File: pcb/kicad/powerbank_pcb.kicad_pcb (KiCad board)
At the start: 2 copper layers, 17.9 x 64.9 mm, 32 parts, among them J1 USB_C_OUT, J2 USB_C_IN, U1 TPS61022, U2 IP2312-ESOP8

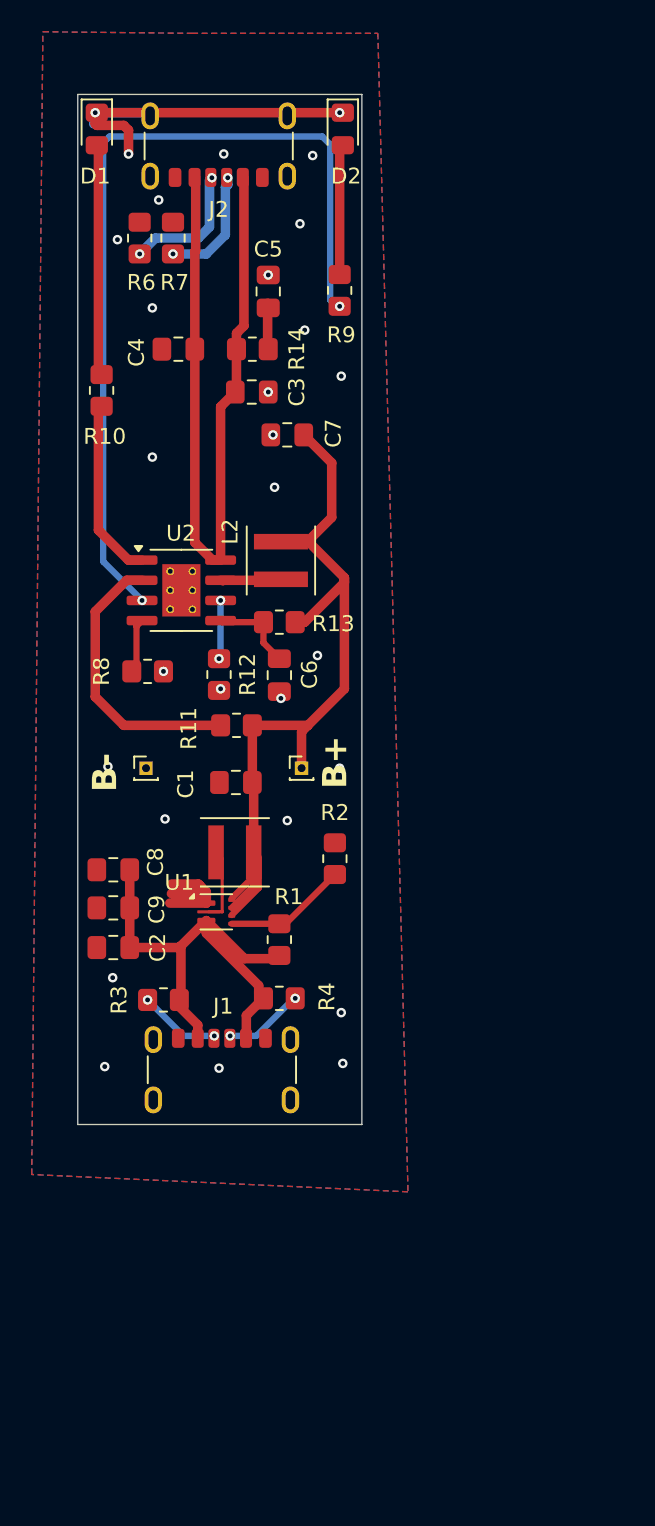
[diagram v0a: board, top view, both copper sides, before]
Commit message: first draft
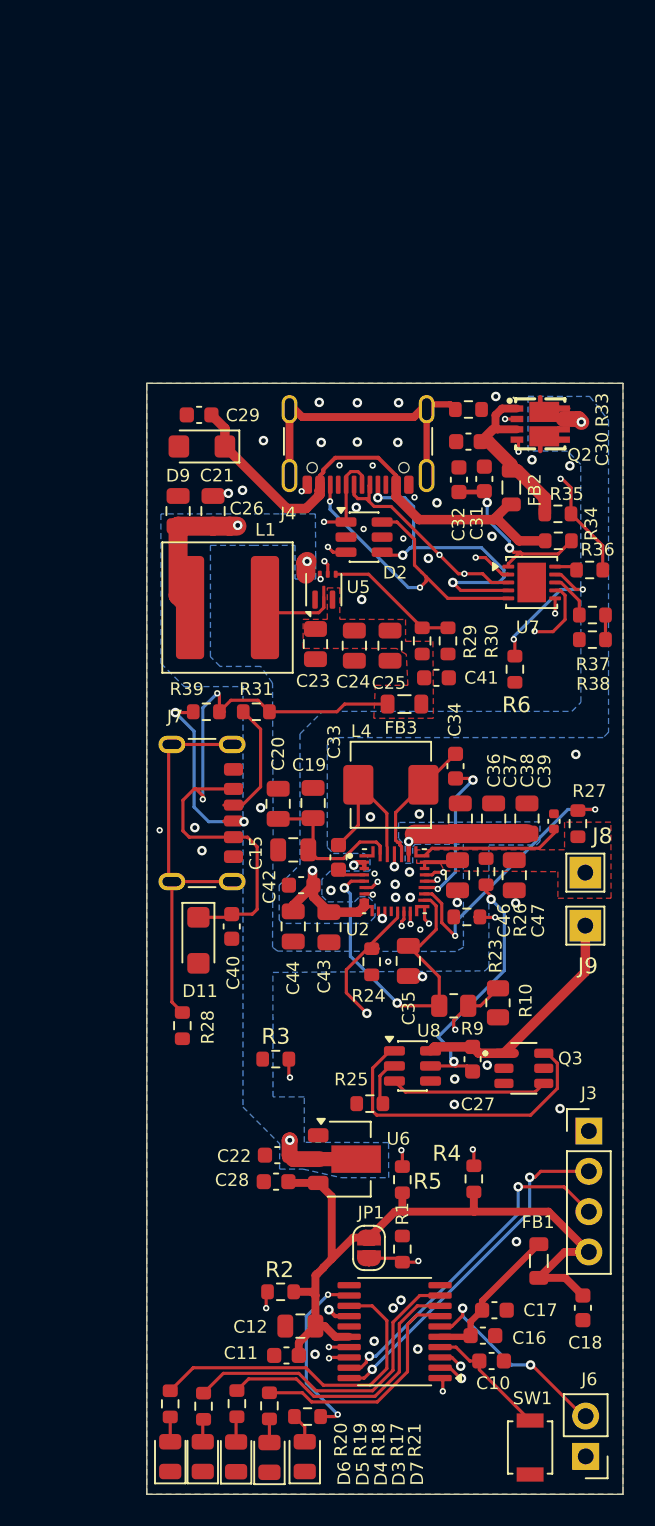
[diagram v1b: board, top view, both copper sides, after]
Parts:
- removed C1, C4, C5: 10uF, Capacitor_SMD:C_0805_2012Metric_Pad1.18x1.45mm_HandSolder
- removed C2, C3, C6, C7, C8, C9: 22uF, Capacitor_SMD:C_0805_2012Metric_Pad1.18x1.45mm_HandSolder
- removed D1: LED_RED, LED_SMD:LED_0805_2012Metric_Pad1.15x1.40mm_HandSolder
- removed J1: USB_C_OUT, Connector_USB:USB_C_Receptacle_GCT_USB4125-xx-x_6P_TopMnt_Horizontal
- removed J2: USB_C_IN, Connector_USB:USB_C_Receptacle_GCT_USB4125-xx-x_6P_TopMnt_Horizontal
- removed L2: 1uH, Inductor_SMD:L_Coilcraft_XxL4030
- removed R11: 1k, Resistor_SMD:R_0805_2012Metric_Pad1.20x1.40mm_HandSolder
- removed R12: 45k, Resistor_SMD:R_0805_2012Metric_Pad1.20x1.40mm_HandSolder
- removed R13: 0.5R, Resistor_SMD:R_0805_2012Metric_Pad1.20x1.40mm_HandSolder
- removed R14: 2R, Resistor_SMD:R_0805_2012Metric_Pad1.20x1.40mm_HandSolder
- removed R7: 5.1k, Resistor_SMD:R_0805_2012Metric_Pad1.20x1.40mm_HandSolder
- removed R8: 51k, Resistor_SMD:R_0805_2012Metric_Pad1.20x1.40mm_HandSolder
- removed REF** (x2): PinHeader_1x01_P1.00mm_Vertical, Connector_PinHeader_1.00mm:PinHeader_1x01_P1.00mm_Vertical
- added C10: 100n, Capacitor_SMD:C_0603_1608Metric, F.Cu at (93.4, 126.8)
- added C11: 100n, Capacitor_SMD:C_0603_1608Metric, F.Cu at (80.5, 126.4)
- added C12: 10u, Capacitor_SMD:C_0805_2012Metric, F.Cu at (81.3, 124.5)
- added C15: 100n, Capacitor_SMD:C_0805_2012Metric, F.Cu at (80.9, 94.5)
- added C16: 10n, Capacitor_SMD:C_0603_1608Metric, F.Cu at (92.8, 125.2)
- added C17: 1u, Capacitor_SMD:C_0603_1608Metric, F.Cu at (93.5, 123.5)
- added C18: 1u, Capacitor_SMD:C_0603_1608Metric, F.Cu at (99.1, 123.4)
- added C19: 47u, Capacitor_SMD:C_0805_2012Metric, F.Cu at (82.1, 91.6)
- added C20: 47u, Capacitor_SMD:C_0805_2012Metric, F.Cu at (79.9, 91.6)
- added C21: 10uF, Capacitor_SMD:C_0805_2012Metric, F.Cu at (75.8, 73.2)
- added C22: 1u, Capacitor_SMD:C_0603_1608Metric, F.Cu at (79.9, 113.8)
- added C23: 22uF, Capacitor_SMD:C_0805_2012Metric, F.Cu at (82.3, 81.6)
- added C24: 22uF, Capacitor_SMD:C_0805_2012Metric, F.Cu at (84.7, 81.7)
- added C25: 22uF, Capacitor_SMD:C_0805_2012Metric, F.Cu at (87.0, 81.7)
- added C26: 10uF, Capacitor_SMD:C_0805_2012Metric, F.Cu at (73.6, 73.2)
- added C27: 0.1uF, Capacitor_SMD:C_0603_1608Metric, F.Cu at (92.2, 107.7)
- added C28: 1u, Capacitor_SMD:C_0603_1608Metric, F.Cu at (79.8, 115.5)
- added C29: 2.2u, Capacitor_SMD:C_0603_1608Metric, F.Cu at (74.9, 67.1)
- added C30: 2.2u, Capacitor_SMD:C_0603_1608Metric, F.Cu at (91.9, 68.8)
- added C31: 1u, Capacitor_SMD:C_0603_1608Metric, F.Cu at (92.9, 71.2)
- added C32: 100n, Capacitor_SMD:C_0603_1608Metric, F.Cu at (91.3, 71.2)
- added C33: 47n, Capacitor_SMD:C_0603_1608Metric, F.Cu at (83.7, 95.0)
- added C34: 47n, Capacitor_SMD:C_0603_1608Metric, F.Cu at (91.1, 89.3)
- added C35: 10u, Capacitor_SMD:C_0805_2012Metric, F.Cu at (88.1, 101.5)
- added C36: 100n, Capacitor_SMD:C_0805_2012Metric, F.Cu at (91.4, 92.6)
- added C37: 47u, Capacitor_SMD:C_0805_2012Metric, F.Cu at (93.5, 92.6)
- added C38: 47u, Capacitor_SMD:C_0805_2012Metric, F.Cu at (95.6, 92.6)
- added C39: 1n, Capacitor_SMD:C_0402_1005Metric, F.Cu at (97.3, 92.8)
- added C40: 2.2u, Capacitor_SMD:C_0603_1608Metric, F.Cu at (77.0, 99.4)
- added C41: 2.2u, Capacitor_SMD:C_0603_1608Metric, F.Cu at (89.9, 83.7)
- added C42: 100n, Capacitor_SMD:C_0603_1608Metric, F.Cu at (81.4, 96.8)
- added C43: 10u, Capacitor_SMD:C_0805_2012Metric, F.Cu at (83.1, 99.4)
- added C44: 10u, Capacitor_SMD:C_0805_2012Metric, F.Cu at (80.9, 99.4)
- added C46: 10u, Capacitor_SMD:C_0805_2012Metric, F.Cu at (91.2, 96.1)
- added C47: 10u, Capacitor_SMD:C_0805_2012Metric, F.Cu at (94.8, 96.1)
- added D11: SMF20A, Diode_SMD:D_SMF, F.Cu at (74.9, 100.2)
- added D3: LED, LED_SMD:LED_0805_2012Metric, F.Cu at (79.4, 132.8)
- added D4: LED, LED_SMD:LED_0805_2012Metric, F.Cu at (77.3, 132.8)
- added D5: LED, LED_SMD:LED_0805_2012Metric, F.Cu at (75.2, 132.8)
- added D6: LED, LED_SMD:LED_0805_2012Metric, F.Cu at (73.1, 132.8)
- added D7: LED, LED_SMD:LED_0805_2012Metric, F.Cu at (81.6, 132.8)
- added D9: SMF20A, Diode_SMD:D_SMF, F.Cu at (75.1, 69.1)
- added FB1: 120R, Inductor_SMD:L_0805_2012Metric, F.Cu at (96.3, 120.5)
- added FB2: 8A, Inductor_SMD:L_0805_2012Metric, F.Cu at (94.6, 71.7)
- added FB3: 8A, Inductor_SMD:L_0805_2012Metric, F.Cu at (87.9, 85.4)
- added J3: Conn_01x04_Pin, Connector_PinHeader_2.54mm:PinHeader_1x04_P2.54mm_Vertical, F.Cu at (99.5, 112.3)
- added J4: USB_C_Receptacle_USB2.0_14P, Connector_USB:USB_C_Receptacle_GCT_USB4105-xx-A_16P_TopMnt_Horizontal, F.Cu at (85.0, 67.9)
- added J6: Switch_Conn, Connector_PinHeader_2.54mm:PinHeader_1x02_P2.54mm_Vertical, F.Cu at (99.3, 132.8)
- added J7: USB_C_OUT, Connector_USB:USB_C_Receptacle_GCT_USB4125-xx-x_6P_TopMnt_Horizontal, F.Cu at (74.0, 92.2)
- added J8: Conn_01x01, TestPoint:TestPoint_THTPad_2.0x2.0mm_Drill1.0mm, F.Cu at (99.3, 96.0)
- added J9: Conn_01x01, TestPoint:TestPoint_THTPad_2.0x2.0mm_Drill1.0mm, F.Cu at (99.3, 99.3)
- added JP1: SolderJumper, Jumper:SolderJumper-2_P1.3mm_Open_RoundedPad1.0x1.5mm, F.Cu at (85.7, 119.6)
- added L4: 1u, Inductor_SMD:L_Changjiang_FXL0530, F.Cu at (87.0, 90.4)
- added Q2: SI7223DN-T1-GE3, si7223dn:PDFN3333-8_L3.1-W3.1-P0.65-LS3.4-BL-EP, F.Cu at (96.4, 67.7)
- added Q3: FS8205, FS8205:SOT95P280X145-6N, F.Cu at (95.4, 108.3)
- added R17: 1.5k, Resistor_SMD:R_0603_1608Metric, F.Cu at (79.4, 129.6)
- added R18: 1.5k, Resistor_SMD:R_0603_1608Metric, F.Cu at (77.3, 129.4)
- added R19: 1.5k, Resistor_SMD:R_0603_1608Metric, F.Cu at (75.2, 129.6)
- added R20: 1.5k, Resistor_SMD:R_0603_1608Metric, F.Cu at (73.1, 129.4)
- added R21: 1.5k, Resistor_SMD:R_0603_1608Metric, F.Cu at (81.8, 130.2)
- added R23: 3.0k, Resistor_SMD:R_0603_1608Metric, F.Cu at (91.8, 98.8)
- added R24: 1M, Resistor_SMD:R_0603_1608Metric, F.Cu at (85.8, 101.6)
- added R25: 1k, Resistor_SMD:R_0603_1608Metric, F.Cu at (85.7, 110.5)
- added R26: 100, Resistor_SMD:R_0603_1608Metric, F.Cu at (93.0, 95.9)
- added R27: 100, Resistor_SMD:R_0603_1608Metric, F.Cu at (98.8, 92.9)
- added R28: 1M, Resistor_SMD:R_0603_1608Metric, F.Cu at (73.9, 105.6)
- added R29: 732k, Resistor_SMD:R_0603_1608Metric, F.Cu at (89.0, 81.4)
- added R30: 100k, Resistor_SMD:R_0603_1608Metric, F.Cu at (90.6, 81.4)
- added R31: 10k, Resistor_SMD:R_0603_1608Metric, F.Cu at (78.5, 85.8)
- added R33: 1M, Resistor_SMD:R_0603_1608Metric, F.Cu at (91.9, 66.8)
- added R34: 10, Resistor_SMD:R_0603_1608Metric, F.Cu at (97.6, 75.1)
- added R35: 49.9k, Resistor_SMD:R_0603_1608Metric, F.Cu at (97.5, 73.4)
- added R36: 5.1k, Resistor_SMD:R_0603_1608Metric, F.Cu at (99.5, 76.9)
- added R37: 5.6k, Resistor_SMD:R_0603_1608Metric, F.Cu at (99.7, 79.8)
- added R38: 470, Resistor_SMD:R_0603_1608Metric, F.Cu at (99.7, 81.3)
- added R39: 10k, Resistor_SMD:R_0603_1608Metric, F.Cu at (75.4, 85.8)
- added R5: 10k, Resistor_SMD:R_0603_1608Metric, F.Cu at (87.8, 115.3)
- added SW1: SW_Push, Button_Switch_SMD:SW_SPST_B3U-1000P, F.Cu at (95.8, 132.2)
- added U5: TPS61022, Package_DFN_QFN:Texas_RWU0007A_VQFN-7_2x2mm_P0.5mm, F.Cu at (82.8, 78.2)
- added U6: MCP1700x-330xxMB, Package_TO_SOT_SMD:SOT-89-3, F.Cu at (84.4, 114.0)
- added U7: HUSB238_xxxDD, Package_DFN_QFN:WDFN-10-1EP_3x3mm_P0.5mm_EP1.8x2.5mm, F.Cu at (95.9, 77.7)
- added U8: DW01A, Package_TO_SOT_SMD:SOT-23-6, F.Cu at (88.4, 108.2)
- D2: value LED_BLUE -> SMF05CT1G; footprint LED_SMD:LED_0805_2012Metric_Pad1.15x1.40mm_HandSolder -> Package_TO_SOT_SMD:SOT-23-6
- L1: footprint Inductor_SMD:L_Coilcraft_XxL4030 -> Inductor_SMD:L_Coilcraft_XAL7030-102
- R1: value 732k -> 10k; footprint Resistor_SMD:R_0805_2012Metric_Pad1.20x1.40mm_HandSolder -> Resistor_SMD:R_0603_1608Metric
- R10, R9: value 500R -> 10k; footprint Resistor_SMD:R_0805_2012Metric_Pad1.20x1.40mm_HandSolder -> Resistor_SMD:R_0805_2012Metric
- R2: value 100k -> 10k; footprint Resistor_SMD:R_0805_2012Metric_Pad1.20x1.40mm_HandSolder -> Resistor_SMD:R_0603_1608Metric
- R3: value 10k -> 100k; footprint Resistor_SMD:R_0805_2012Metric_Pad1.20x1.40mm_HandSolder -> Resistor_SMD:R_0603_1608Metric
- R4: footprint Resistor_SMD:R_0805_2012Metric_Pad1.20x1.40mm_HandSolder -> Resistor_SMD:R_0603_1608Metric
- R6: value 5.1k -> 22.6k; footprint Resistor_SMD:R_0805_2012Metric_Pad1.20x1.40mm_HandSolder -> Resistor_SMD:R_0603_1608Metric
- U1: value TPS61022 -> STM32L011F4Px; footprint Package_DFN_QFN:Texas_RWU0007A_VQFN-7_2x2mm_P0.5mm -> Package_SO:TSSOP-20_4.4x6.5mm_P0.65mm
- U2: value IP2312-ESOP8 -> BQ25672RQMR; footprint Package_SO:SOIC-8-1EP_3.9x4.9mm_P1.27mm_EP2.41x3.3mm_ThermalVias -> BQ25672RQMR:IC_BQ25672RQMR
- moved R10 46.0 mm to (93.8, 104.2)
- moved R9 45.6 mm to (91.0, 104.4), turned to 180 degrees
- moved R6 36.0 mm to (94.8, 83.2), turned to -90 degrees
- moved U1 28.7 mm to (87.3, 124.9), turned to 180 degrees
- moved R2 27.5 mm to (80.1, 122.4), turned to 180 degrees
- moved D2 25.7 mm to (85.3, 74.8), turned to 0 degrees
- moved U2 22.7 mm to (87.2, 96.5)
- moved R1 21.0 mm to (87.8, 119.7)
- moved R4 16.7 mm to (92.3, 115.3), turned to 90 degrees
- moved L1 15.4 mm to (76.7, 79.3), turned to 0 degrees
- moved R3 8.00 mm to (79.8, 107.7)
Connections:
- D2 pad 1: GND -> /USB_D+
- D2 pad 2: Net-(D2-A) -> GND
- L1 pad 1: +BATT -> /VSYS
- L1 pad 2: Net-(U1-SW) -> Net-(U5-SW)
- R1 pad 1: Net-(U1-FB) -> GND
- R1 pad 2: Net-(U1-VOUT) -> Net-(JP1-B)
- R10 pad 1: Net-(U2-LED1) -> GND
- R10 pad 2: Net-(D1-A) -> /TS
- R2 pad 1: GND -> +3.3V
- R2 pad 2: Net-(U1-FB) -> /SCL
- R3 pad 1: Net-(J1-CC1) -> GND
- R3 pad 2: Net-(U1-VOUT) -> EN
- R4 pad 1: Net-(J1-CC2) -> +3.3V
- R4 pad 2: Net-(U1-VOUT) -> /INT
- R9 pad 1: Net-(U2-LED2) -> /TS
- R9 pad 2: Net-(D2-A) -> /REGN
- U1 pad 1: GND -> Net-(JP1-B)
- U1 pad 2: Net-(U1-SW) -> /CE
- U1 pad 3: Net-(U1-VOUT) -> /INT
- U1 pad 4: Net-(U1-FB) -> Net-(U1-NRST)
- U1 pad 5: +BATT -> +3.3VA
- U1 pad 6: +BATT -> Net-(J6-Pin_2)
- U1 pad 7: +BATT -> Net-(U1-PA1)
- U2 pad 1: Net-(U2-LED1) -> unconnected-(U2-STAT-Pad1)
- U2 pad 2: Net-(U2-Test) -> /VBUS
- U2 pad 3: Net-(U2-LED2) -> /VBUS
- U2 pad 5: Net-(U2-BAT) -> /REGN
- U2 pad 6: Net-(U2-ICHG) -> /USB_D+
- U2 pad 7: Net-(U2-SW) -> /USB_D-
- U2 pad 8: Net-(U2-VIN) -> /VBUS
- U2 pad 9: GND -> /VBUS
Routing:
- net /SCL: track 0.00 -> 64.3 mm, vias 0 -> 4
- net /SDA: track 0.00 -> 63.3 mm, vias 0 -> 4
- net Net-(U2-LED2): track 54.7 -> 0.00 mm, vias 2 -> 0
- net +BATT: track 54.2 -> 0.00 mm
- net EN: track 0.00 -> 53.1 mm, vias 0 -> 3
- net Net-(U2-VIN): track 49.9 -> 0.00 mm
- net /USB_D-: track 0.00 -> 48.3 mm, vias 0 -> 4
- net +3.3V: track 0.00 -> 46.0 mm
- net /USB_D+: track 0.00 -> 43.4 mm, vias 0 -> 3
- net /INT: track 0.00 -> 39.9 mm, vias 0 -> 3
- net Net-(D11-A1): track 0.00 -> 38.9 mm, vias 0 -> 2
- net /CE: track 0.00 -> 35.8 mm, vias 0 -> 2
- net GND: track 32.3 -> 0.00 mm, vias 29 -> 54
- net Net-(U1-VOUT): track 32.1 -> 0.00 mm
- net /USB_VBUS_PRE: track 0.00 -> 31.5 mm
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- added copper zone on B.Cu, net /VBUS
- added copper zone on F.Cu, net /VOUT
- added copper zone on B.Cu, net /VSYS
- added copper zone on F.Cu, net BAT
- added copper zone on In1.Cu, net GND
- added copper zone on In2.Cu, net GND
- removed copper zone on B.Cu, net GND
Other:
- board size 17.9 x 64.9 mm -> 30 x 70 mm
- copper layers 2 -> 4
- board text added: "Tessy"
- board text removed: "B+"
- board text removed: "B-"
- board text removed: "DESIGNED AND ASSEMBLED IN GERMANY"
- board text removed: "FL@NK POWERBANK"
- board text removed: "JLCJLCJLCJLC"
- board text removed: "github.com/k-off/powerbank pacovali@student.42berlin.de"
